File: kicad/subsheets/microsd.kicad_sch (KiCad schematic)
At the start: 21 parts, among them Q1 FDN340P

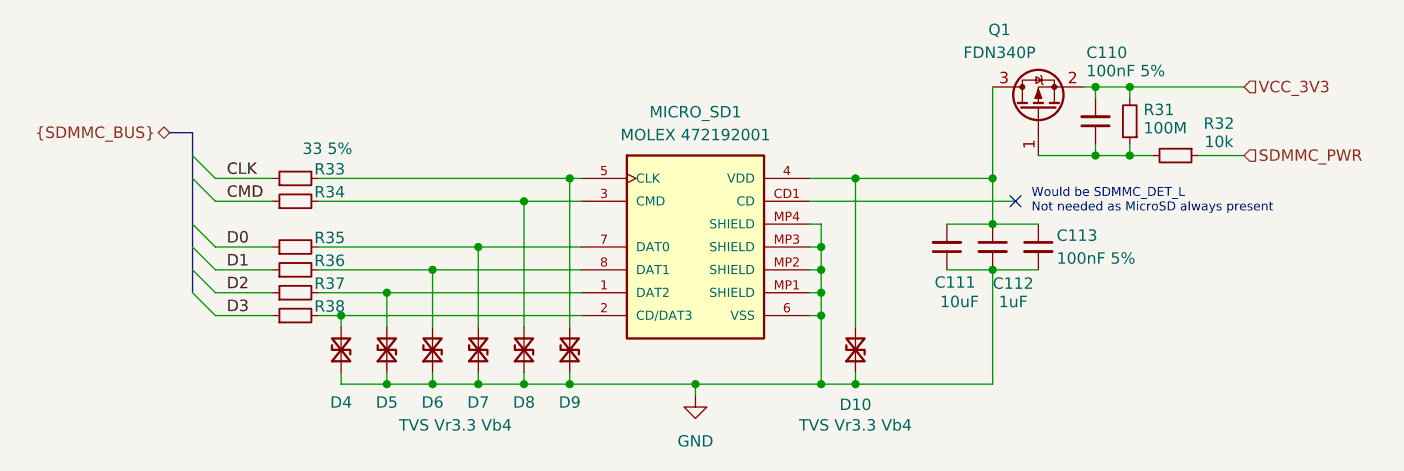
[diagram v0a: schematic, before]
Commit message: Annotations + minor tweaks
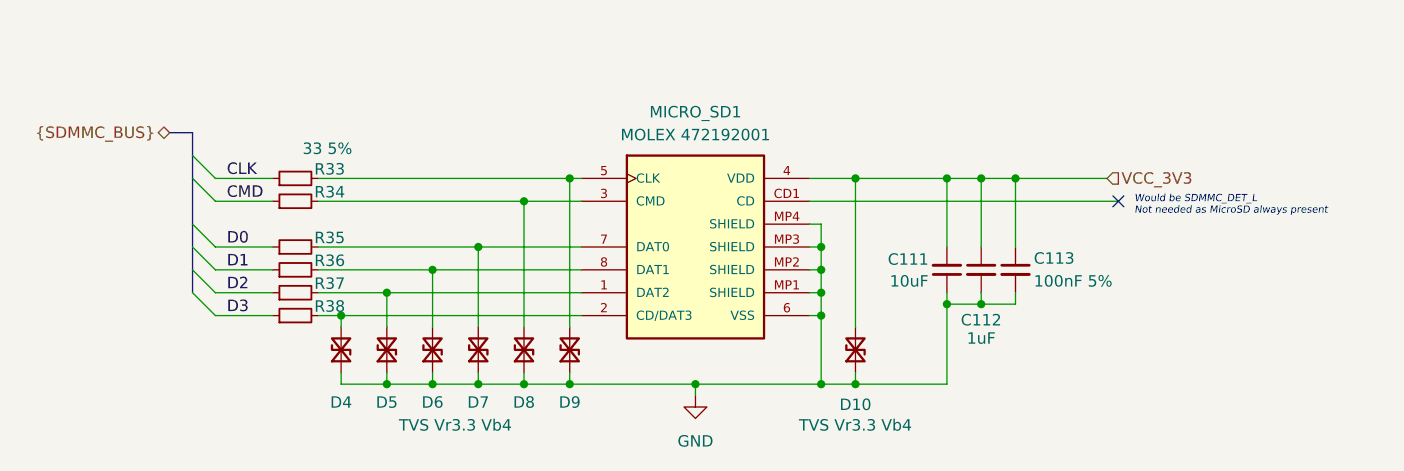
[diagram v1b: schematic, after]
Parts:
- removed C110: 100nF 5%, Capacitor_SMD:C_0201_0603Metric, symbol Device:C_Small
- removed Q1: FDN340P, Package_TO_SOT_SMD:SOT-23, symbol Transistor_FET:FDN340P
- removed R31: 100M, Resistor_SMD:R_0603_1608Metric, symbol Device:R_Small
- removed R32: 10k, Resistor_SMD:R_0603_1608Metric, symbol Device:R_Small
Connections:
- net VCC_3V3: now also C111.2, C112.1, C113.1, D10.2 (A2), MICRO_SD1.4 (VDD)
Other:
- moved on the sheet: C111, C112, C113
